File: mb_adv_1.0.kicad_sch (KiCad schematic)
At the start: 5 parts, among them SW2 SW_SP3T, U2 gba_link_cable, U3 BOB-12009

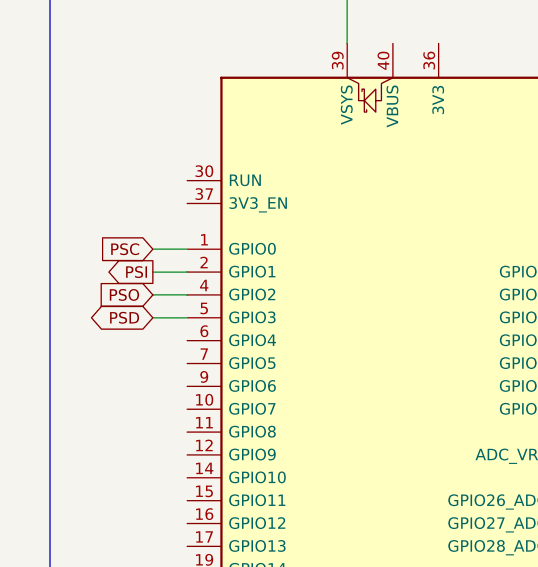
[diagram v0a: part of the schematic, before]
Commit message: update README.md, schematic, and pcb
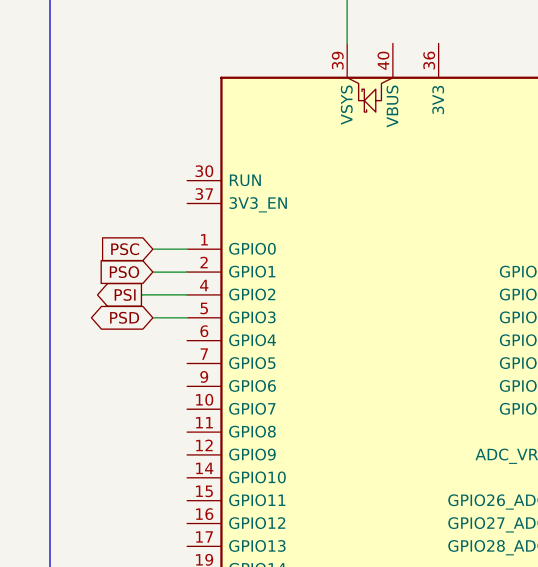
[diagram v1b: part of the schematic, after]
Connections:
- net PSI: now also A1.4 (GPIO2); no longer A1.2 (GPIO1)
- net PSO: now also A1.2 (GPIO1); no longer A1.4 (GPIO2)
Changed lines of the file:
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@@
-	(wire
-		(pts
-			(xy 50.8 80.01) (xy 54.61 80.01)
-		)
-		(stroke
-			(width 0)
-			(type default)
-		)
-	)
 	(wire
 		(pts
@@
 	(wire
 		(pts
+			(xy 49.53 80.01) (xy 54.61 80.01)
+		)
+		(stroke
+			(width 0)
+			(type default)
+		)
+	)
+	(wire
+		(pts
 			(xy 50.8 77.47) (xy 54.61 77.47)
 		)
@@
 		)
 	)
-	(global_label "PSO"
-		(shape input)
-		(at 50.8 80.01 180)
+	(global_label "HV"
+		(shape output)
+		(at 170.18 44.45 0)
+		(fields_autoplaced yes)
+		(effects
+			(font
+				(size 1.27 1.27)
+			)
+			(justify left)
+		)
+		(property "Intersheetrefs" "${INTERSHEET_REFS}"
+			(at 175.5843 44.45 0)
+			(hide yes)
+			(show_name no)
+			(do_not_autoplace no)
+			(effects
+				(font
+					(size 1.27 1.27)
+				)
+				(justify left)
+			)
+		)
+	)
+	(global_label "LV"
+		(shape output)
+		(at 242.57 59.69 0)
+		(fields_autoplaced yes)
+		(effects
+			(font
+				(size 1.27 1.27)
+			)
+			(justify left)
+		)
+		(property "Intersheetrefs" "${INTERSHEET_REFS}"
+			(at 247.6719 59.69 0)
+			(hide yes)
+			(show_name no)
+			(do_not_autoplace no)
+			(effects
+				(font
+					(size 1.27 1.27)
+				)
+				(justify left)
+			)
+		)
+	)
+	(global_label "OPT_2"
+		(shape output)
+		(at 217.17 111.76 0)
+		(fields_autoplaced yes)
+		(effects
+			(font
+				(size 1.27 1.27)
+			)
+			(justify left)
+		)
+		(property "Intersheetrefs" "${INTERSHEET_REFS}"
+			(at 226.3238 111.76 0)
+			(hide yes)
+			(show_name no)
+			(do_not_autoplace no)
+			(effects
+				(font
+					(size 1.27 1.27)
+				)
+				(justify left)
+			)
+		)
+	)
+	(global_label "HV"
+		(shape output)
+		(at 199.39 59.69 180)
 		(fields_autoplaced yes)
 		(effects
@@
 		)
 		(property "Intersheetrefs" "${INTERSHEET_REFS}"
-			(at 44.0048 80.01 0)
+			(at 193.9857 59.69 0)
 			(hide yes)
 			(show_name no)
@@
 		)
 	)
-	(global_label "HV"
-		(shape output)
-		(at 170.18 44.45 0)
-		(fields_autoplaced yes)
-		(effects
-			(font
-				(size 1.27 1.27)
-			)
-			(justify left)
-		)
-		(property "Intersheetrefs" "${INTERSHEET_REFS}"
-			(at 175.5843 44.45 0)
-			(hide yes)
-			(show_name no)
-			(do_not_autoplace no)
-			(effects
-				(font
-					(size 1.27 1.27)
-				)
-				(justify left)
-			)
-		)
-	)
-	(global_label "LV"
-		(shape output)
-		(at 242.57 59.69 0)
-		(fields_autoplaced yes)
-		(effects
-			(font
-				(size 1.27 1.27)
-			)
-			(justify left)
-		)
-		(property "Intersheetrefs" "${INTERSHEET_REFS}"
-			(at 247.6719 59.69 0)
-			(hide yes)
-			(show_name no)
-			(do_not_autoplace no)
-			(effects
-				(font
-					(size 1.27 1.27)
-				)
-				(justify left)
-			)
-		)
-	)
-	(global_label "OPT_2"
-		(shape output)
-		(at 217.17 111.76 0)
-		(fields_autoplaced yes)
-		(effects
-			(font
-				(size 1.27 1.27)
-			)
-			(justify left)
-		)
-		(property "Intersheetrefs" "${INTERSHEET_REFS}"
-			(at 226.3238 111.76 0)
-			(hide yes)
-			(show_name no)
-			(do_not_autoplace no)
-			(effects
-				(font
-					(size 1.27 1.27)
-				)
-				(justify left)
-			)
-		)
-	)
-	(global_label "HV"
-		(shape output)
-		(at 199.39 59.69 180)
+	(global_label "PSI"
+		(shape output)
+		(at 49.53 80.01 180)
 		(fields_autoplaced yes)
 		(effects
@@
 		)
 		(property "Intersheetrefs" "${INTERSHEET_REFS}"
-			(at 193.9857 59.69 0)
-			(hide yes)
-			(show_name no)
-			(do_not_autoplace no)
-			(effects
-				(font
-					(size 1.27 1.27)
-				)
-				(justify right)
-			)
-		)
-	)
-	(global_label "PSI"
-		(shape output)
-		(at 50.8 77.47 180)
-		(fields_autoplaced yes)
-		(effects
-			(font
-				(size 1.27 1.27)
-			)
-			(justify right)
-		)
-		(property "Intersheetrefs" "${INTERSHEET_REFS}"
-			(at 44.7305 77.47 0)
+			(at 43.4605 80.01 0)
 			(hide yes)
 			(show_name no)
@@
 			)
 		)
+	)
+	(global_label "PSO"
+		(shape input)
+		(at 50.8 77.47 180)
+		(fields_autoplaced yes)
+		(effects
+			(font
+				(size 1.27 1.27)
+			)
+			(justify right)
+		)
+		(property "Intersheetrefs" "${INTERSHEET_REFS}"
+			(at 44.0048 77.47 0)
+			(hide yes)
+			(show_name no)
+			(do_not_autoplace no)
+			(effects
+				(font
+					(size 1.27 1.27)
+				)
+				(justify right)
+			)
+		)
